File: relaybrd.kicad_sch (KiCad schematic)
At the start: 16 parts, among them J7 5499922-4, U10 TPS3850H50DRCR

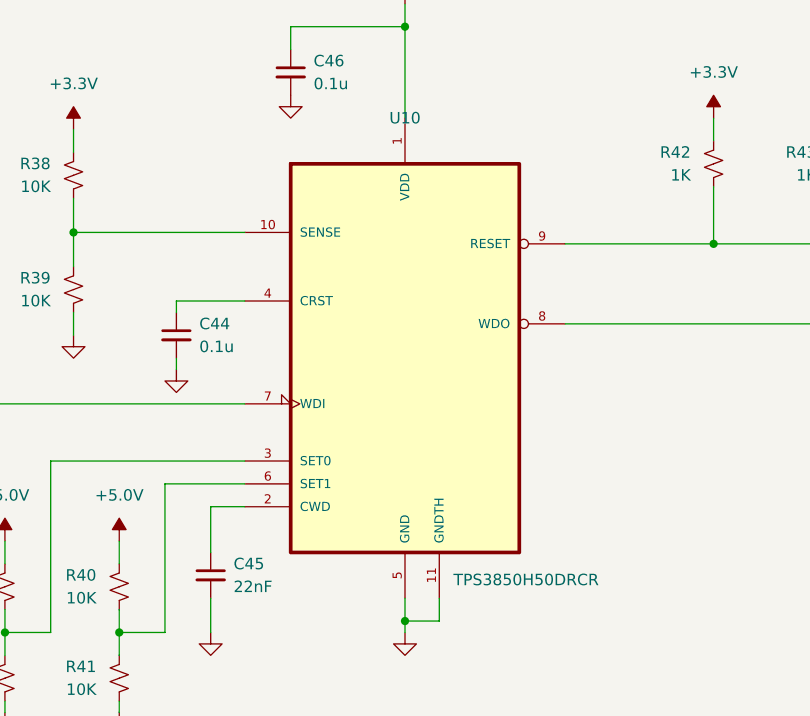
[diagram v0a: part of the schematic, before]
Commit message: Finish BOM
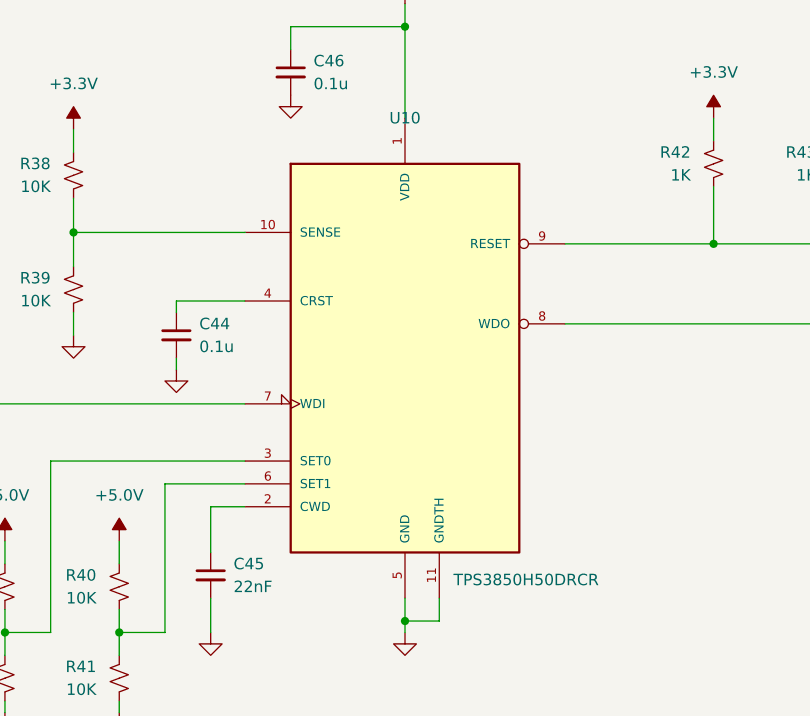
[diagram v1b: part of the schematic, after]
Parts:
- C44, C46: Cost (none) -> .08; MFG (none) -> Taiyo-Yuden; MFG_PN (none) -> TMF212B7104KGHT
- C45: Cost (none) -> .15; MFG (none) -> Kemet; MFG_PN (none) -> C0805C223J3GEC7210
- J7: Cost (none) -> 5.00; MFG (none) -> Molex; MFG_PN (none) -> 5499922-4
- R42, R43: MFG_PN ERJ-2RKF1001X -> ERJ-P06F1001V
- U10: Cost (none) -> 1.85; MFG (none) -> TI
